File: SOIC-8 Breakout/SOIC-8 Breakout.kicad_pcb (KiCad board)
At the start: 2 copper layers, 18 x 15.4 mm, 16 parts

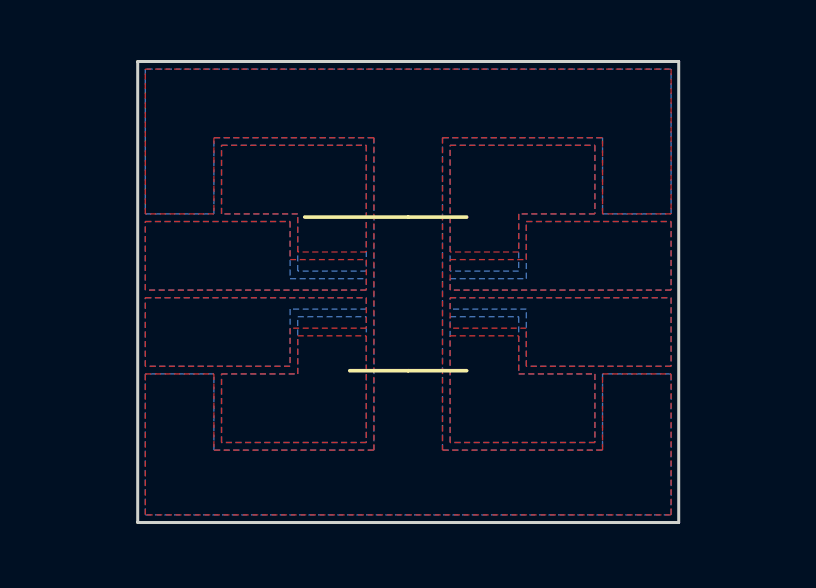
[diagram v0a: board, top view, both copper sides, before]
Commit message: Updated Files
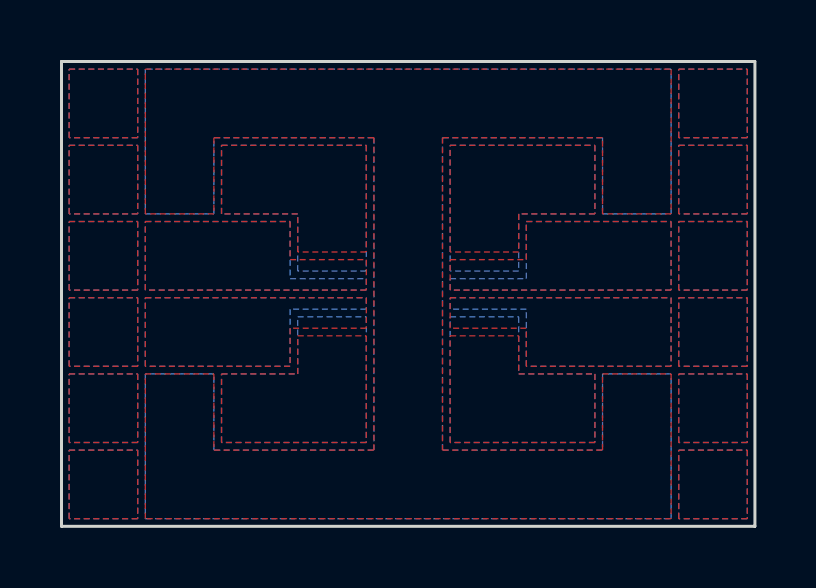
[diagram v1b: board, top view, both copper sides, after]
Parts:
- removed REF**: SOIC-8_3.9x4.9mm_P1.27mm, Package_SO:SOIC-8_3.9x4.9mm_P1.27mm
- removed REF** (x7): C_0402_1005Metric, Capacitor_SMD:C_0402_1005Metric
- removed REF** (x7): C_0603_1608Metric, Capacitor_SMD:C_0603_1608Metric
- removed REF**: MSOP-8_3x3mm_P0.65mm, Package_SO:MSOP-8_3x3mm_P0.65mm
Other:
- board size 18 x 15.4 mm -> 23.1 x 15.5 mm
